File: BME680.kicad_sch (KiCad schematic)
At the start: 20 parts, among them IC1 BME680, Q2 BSS138, U2 AP2112K-3.3

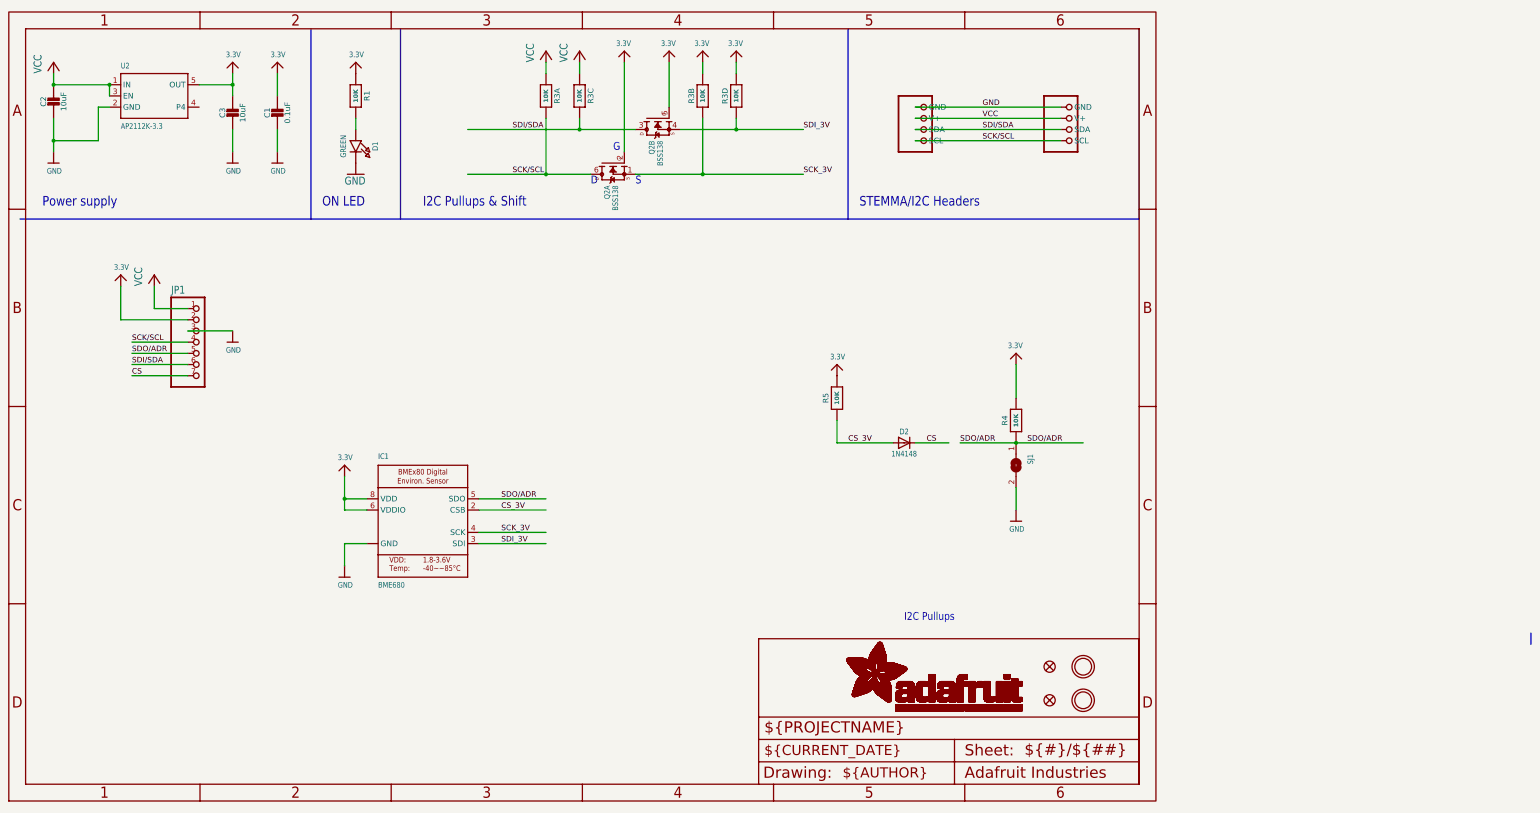
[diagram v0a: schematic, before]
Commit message: added drawing sheet
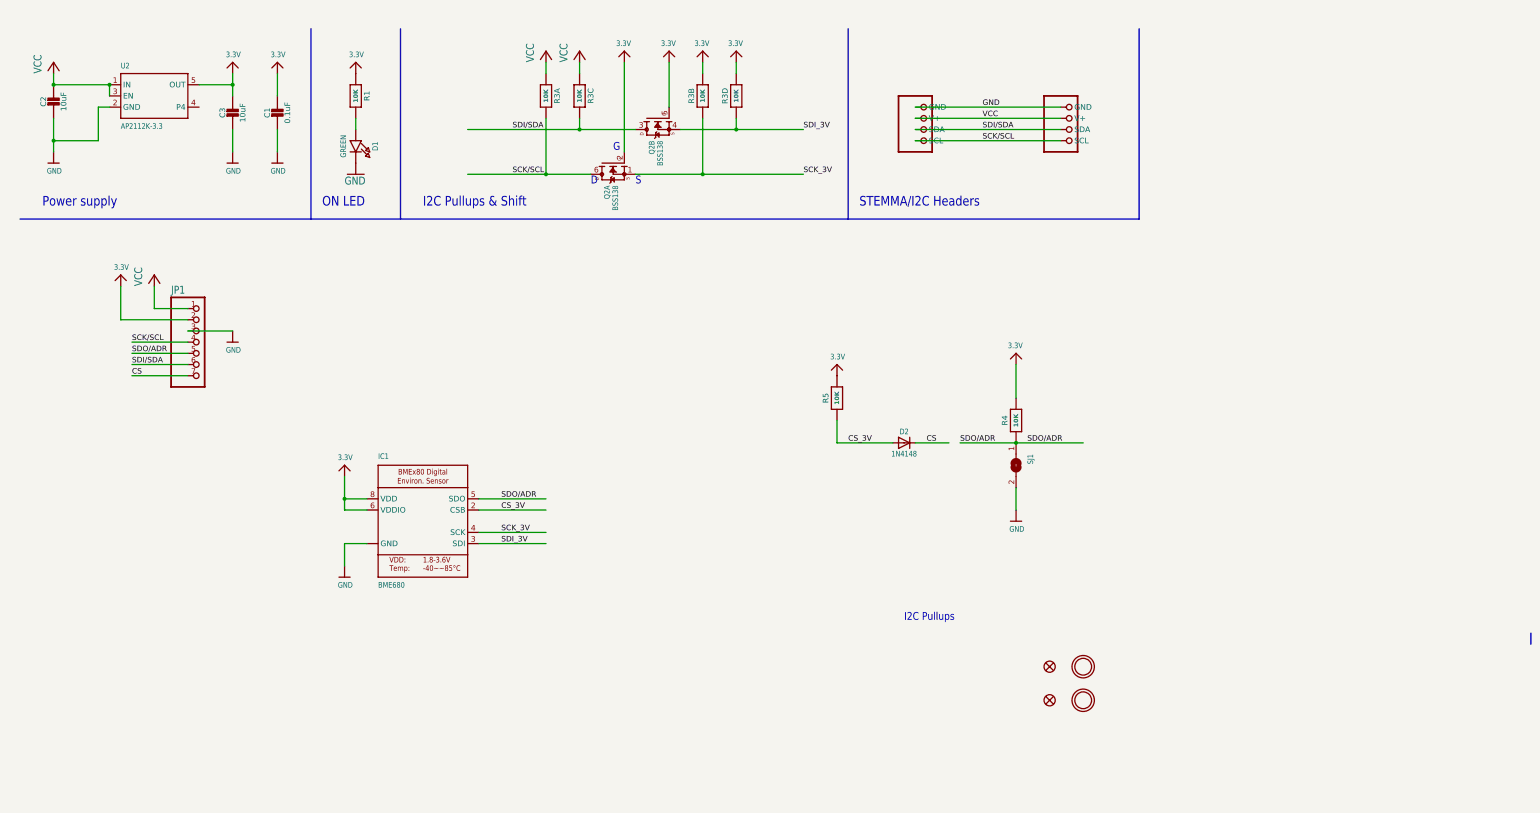
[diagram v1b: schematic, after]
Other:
- title: (none) -> BME680
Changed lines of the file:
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@@
 	(generator "eeschema")
 	(generator_version "8.0")
-	(paper "User" 383.616 217.322)
+	(paper "A4")
+	(title_block
+		(title "BME680")
+		(date "2024-03-06")
+	)
 	(junction
 		(at 175.26 55.88)
@@
 					(unit 1)
 				)
-			)
-		)
-	)
-	(symbol
-		(lib_id "BME680-eagle-import:FRAME_A4_ADAFRUIT")
-		(at 17.78 198.12 0)
-		(unit 1)
-		(exclude_from_sim no)
-		(in_bom yes)
-		(on_board yes)
-		(dnp no)
-		(property "Reference" "#U$18"
-			(at 17.78 198.12 0)
-			(effects
-				(font
-					(size 1.27 1.27)
-				)
-				(hide yes)
-			)
-		)
-		(property "Value" "FRAME_A4_ADAFRUIT"
-			(at 17.78 198.12 0)
-			(effects
-				(font
-					(size 1.27 1.27)
-				)
-				(hide yes)
-			)
-		)
-		(property "Footprint" ""
-			(at 17.78 198.12 0)
-			(effects
-				(font
-					(size 1.27 1.27)
-				)
-				(hide yes)
-			)
-		)
-		(property "Datasheet" ""
-			(at 17.78 198.12 0)
-			(effects
-				(font
-					(size 1.27 1.27)
-				)
-				(hide yes)
-			)
-		)
-		(property "Description" ""
-			(at 17.78 198.12 0)
-			(effects
-				(font
-					(size 1.27 1.27)
-				)
-				(hide yes)
-			)
-		)
-		(instances
-			(project "BME680"
-				(path "/ba694707-55c1-41d4-b2e7-4006a8fc6a7f"
-					(reference "#U$18")
-					(unit 1)
-				)
